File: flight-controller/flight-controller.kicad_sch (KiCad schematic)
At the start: 5 parts, among them J1 Motor_Driver_1, J4 Motor_Driver_2, J5 MD1_5V, J6 MD2_5V, J8 XT60PW-F

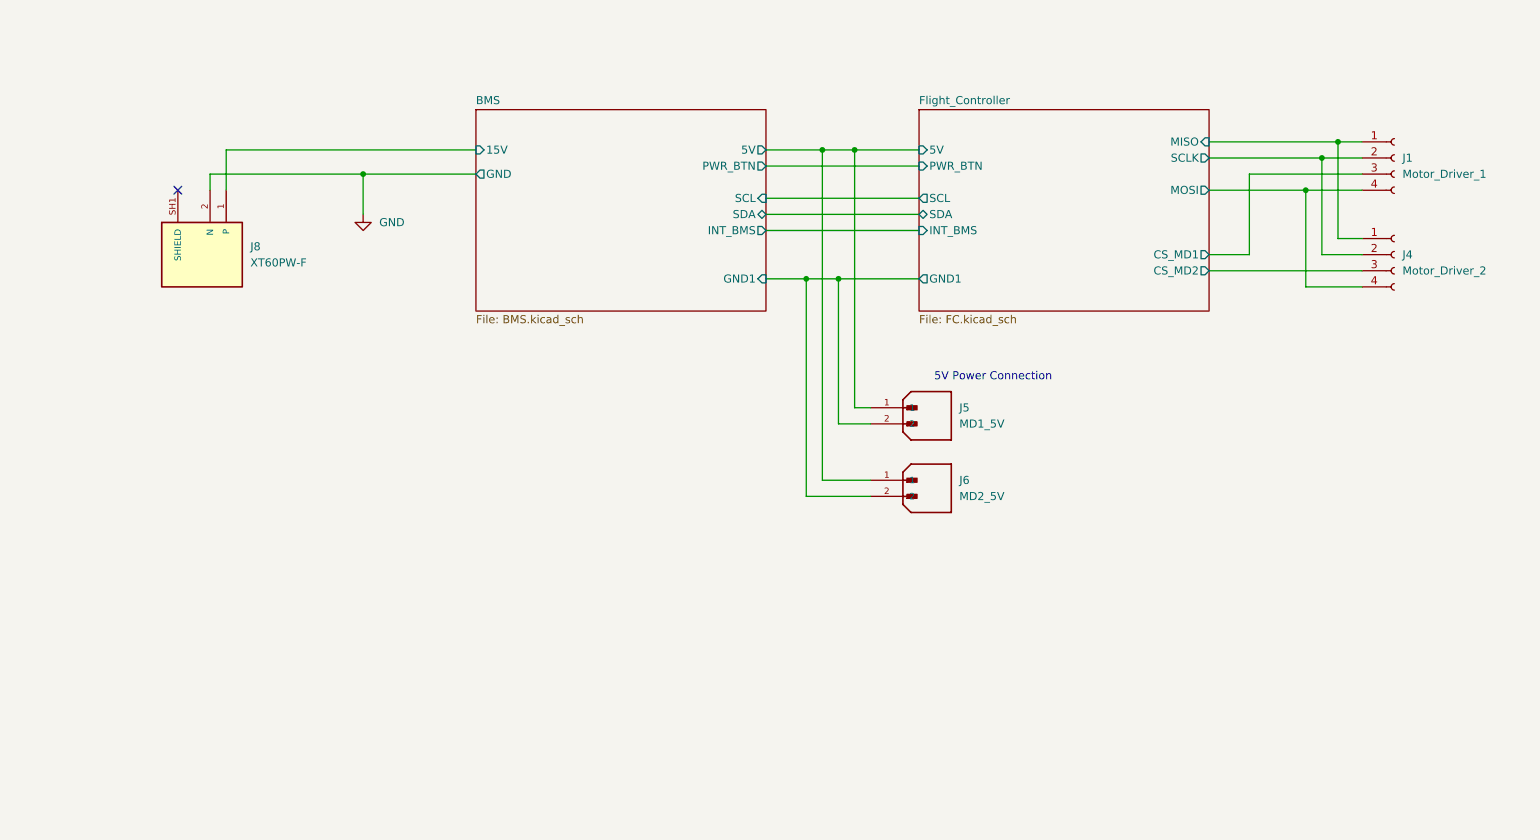
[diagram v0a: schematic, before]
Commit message: cleaned up the layout
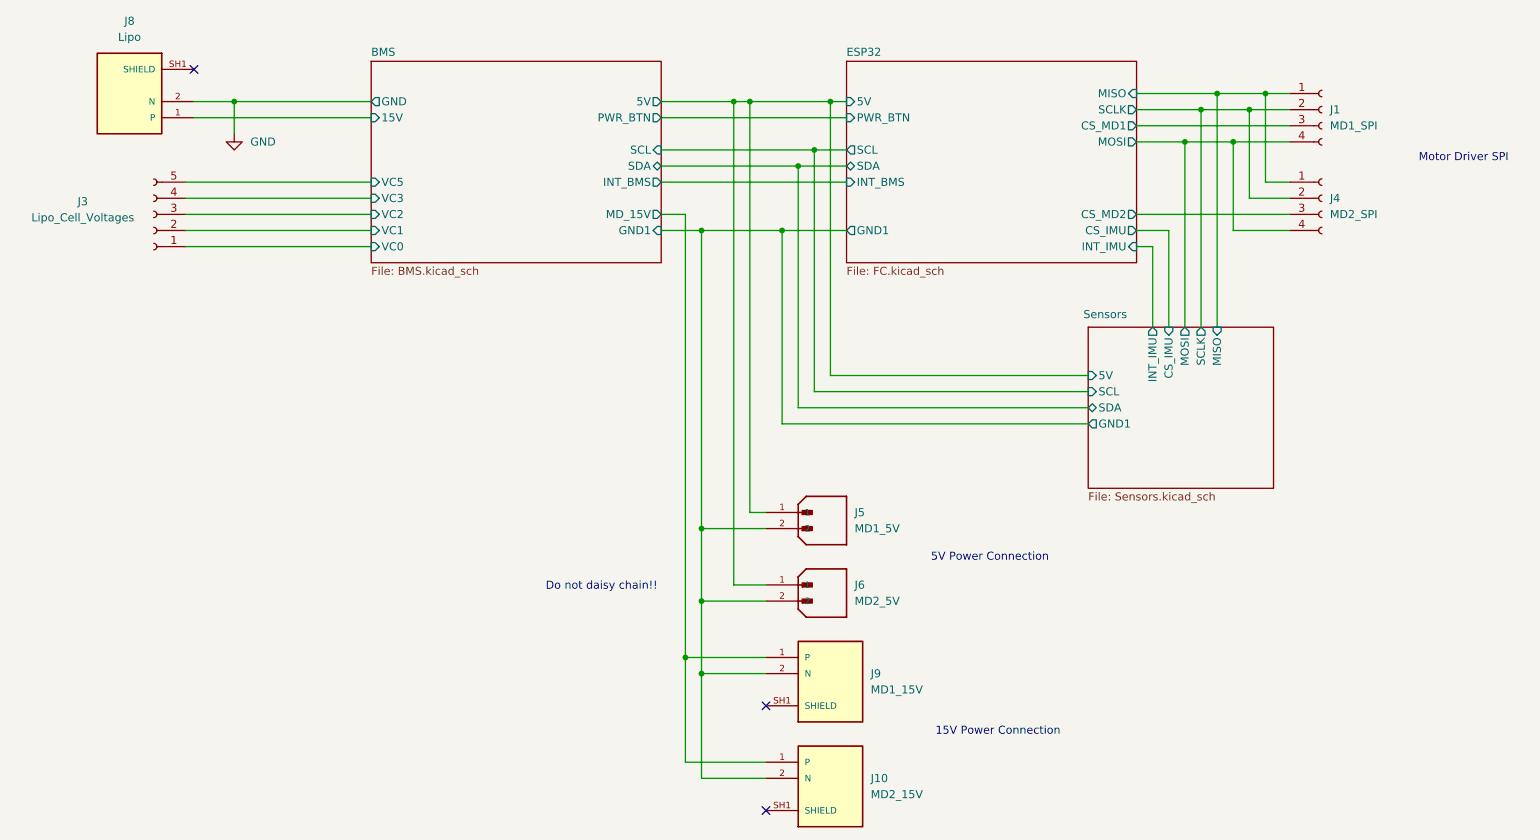
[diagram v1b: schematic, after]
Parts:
- added J10: MD2_15V, Connector_AMASS:AMASS_XT60PW-F_1x02_P7.20mm_Horizontal, symbol XT60PW-F:XT60PW-F
- added J3: Lipo_Cell_Voltages, Connector_JST:JST_XH_S5B-XH-A_1x05_P2.50mm_Horizontal, symbol Connector:Conn_01x05_Socket
- added J9: MD1_15V, Connector_AMASS:AMASS_XT60PW-F_1x02_P7.20mm_Horizontal, symbol XT60PW-F:XT60PW-F
- J1: value Motor_Driver_1 -> MD1_SPI
- J4: value Motor_Driver_2 -> MD2_SPI
- J8: value XT60PW-F -> Lipo
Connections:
- net BMS/GND1: now also J10.2 (N), J9.2 (N)
- new net: J10.SH1 (SHIELD), J10.SH2 (SHIELD)
- new net: J9.SH1 (SHIELD), J9.SH2 (SHIELD)
- new net BMS/MD_15V: J10.1 (P), J9.1 (P)
- new net BMS/VC0: J3.1 (Pin_1)
- new net BMS/VC1: J3.2 (Pin_2)
- new net BMS/VC2: J3.3 (Pin_3)
- new net BMS/VC3: J3.4 (Pin_4)
- new net BMS/VC5: J3.5 (Pin_5)
- no-connect marks 1 -> 3
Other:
- sheet Flight_Controller renamed ESP32
- added sheet Sensors (Sensors.kicad_sch)
- sheet BMS ports: added MD_15V, VC0, VC1, VC2, VC3, VC5; removed none
- sheet ESP32 ports: added CS_IMU, INT_IMU; removed none
- note added: "15V Power Connection"
- note added: "Do not daisy chain!!"
- note added: "Motor Driver SPI"
- moved on the sheet: J1, J4, J5, J6, J8
